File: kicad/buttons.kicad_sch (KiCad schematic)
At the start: 18 parts, among them U4 MAX7219, U6 CD74HC4067M

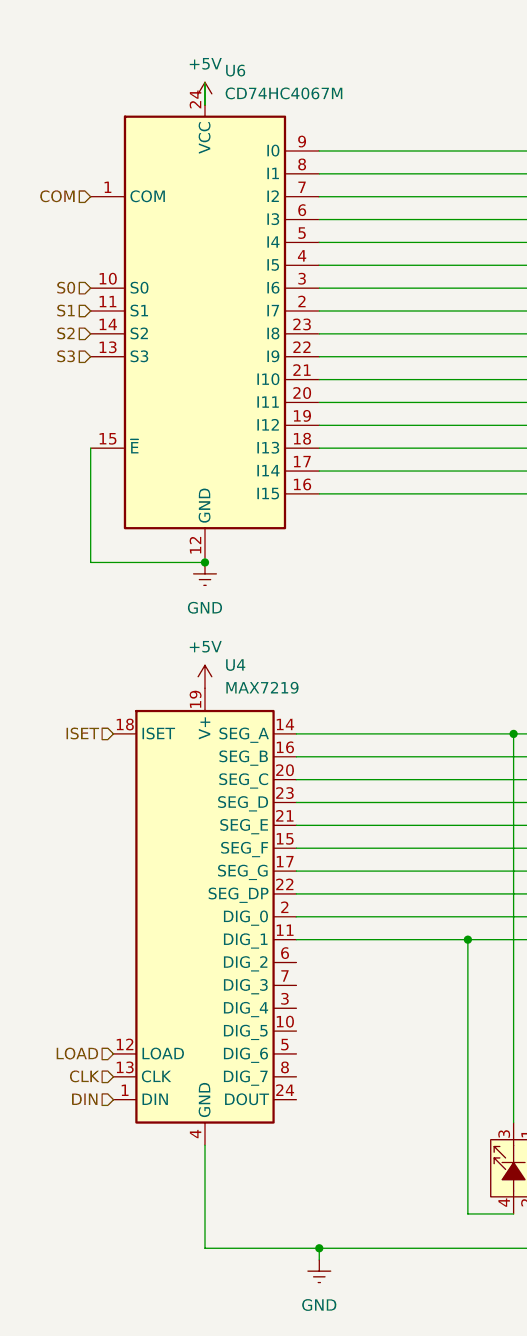
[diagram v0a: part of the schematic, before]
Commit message: kicad updates
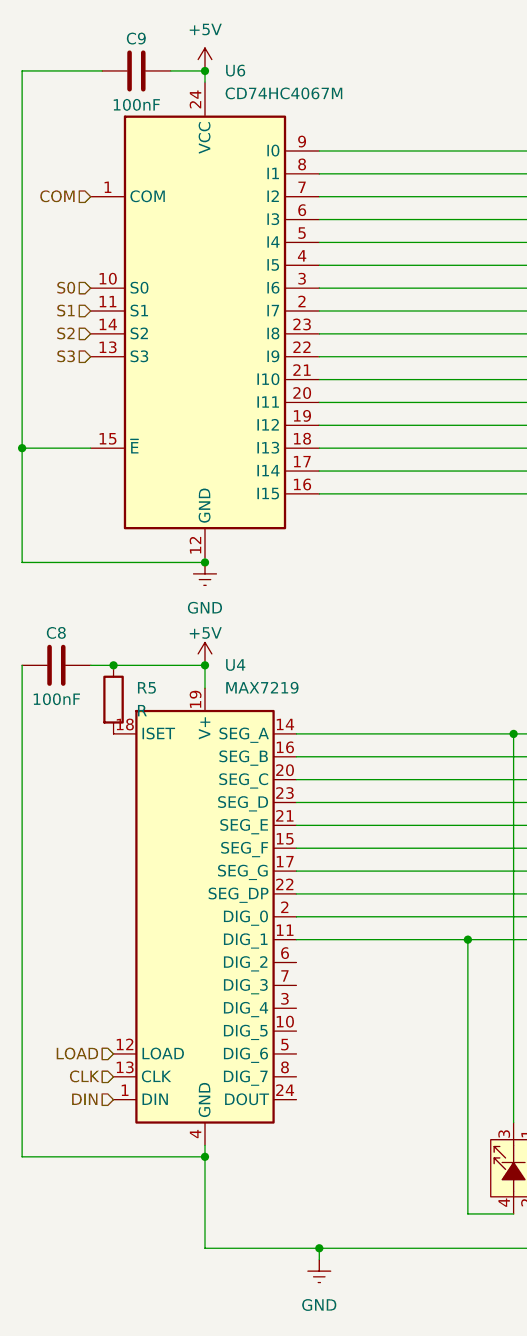
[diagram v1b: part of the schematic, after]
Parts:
- added C8, C9: 100nF, Capacitor_THT:C_Axial_L5.1mm_D3.1mm_P7.50mm_Horizontal, symbol Device:C
- added R5: R, Resistor_THT:R_Axial_DIN0207_L6.3mm_D2.5mm_P10.16mm_Horizontal, symbol Device:R
- U4: footprint (none) -> Package_DIP:DIP-24_W7.62mm_Socket
- mute10, mute11, mute12, mute13, mute14, mute15, mute16, mute9, solo1, solo2, solo3, solo4, solo5, solo6, solo7, solo8: footprint (none) -> mixer:SW_SPST_LED_9mm
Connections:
- net +5V: now also C8.2, C9.2, R5.1
- net GND: now also C8.1, C9.1
- net ISET: no longer names the net of U4.18 (ISET)
- net ISET: now also R5.2
